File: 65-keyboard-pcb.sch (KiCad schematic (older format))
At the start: 67 parts

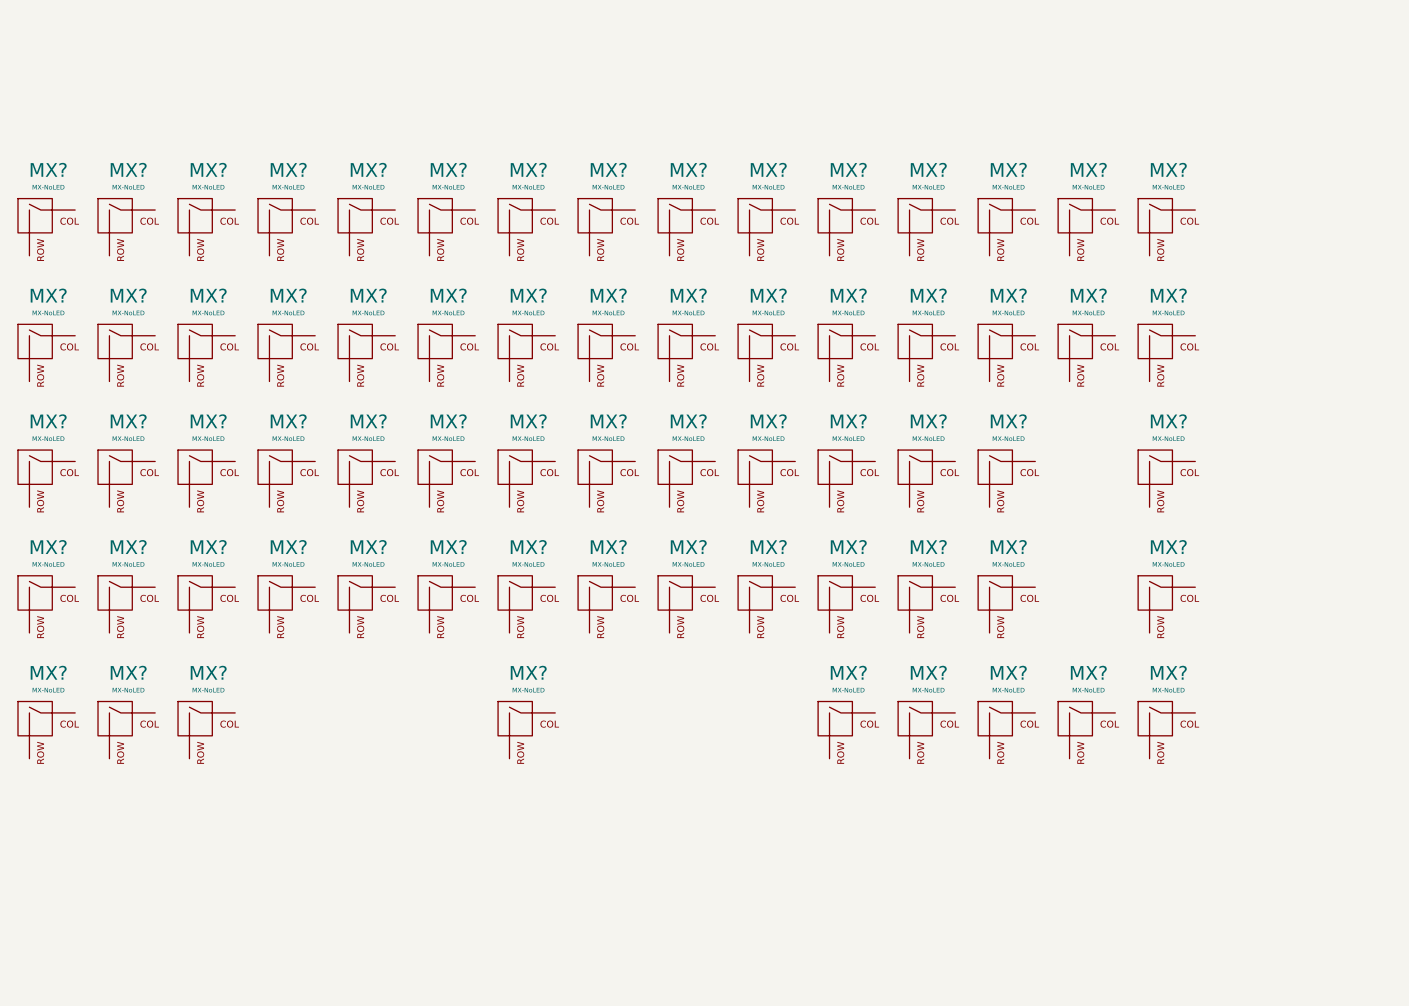
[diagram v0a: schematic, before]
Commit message: Design matrix
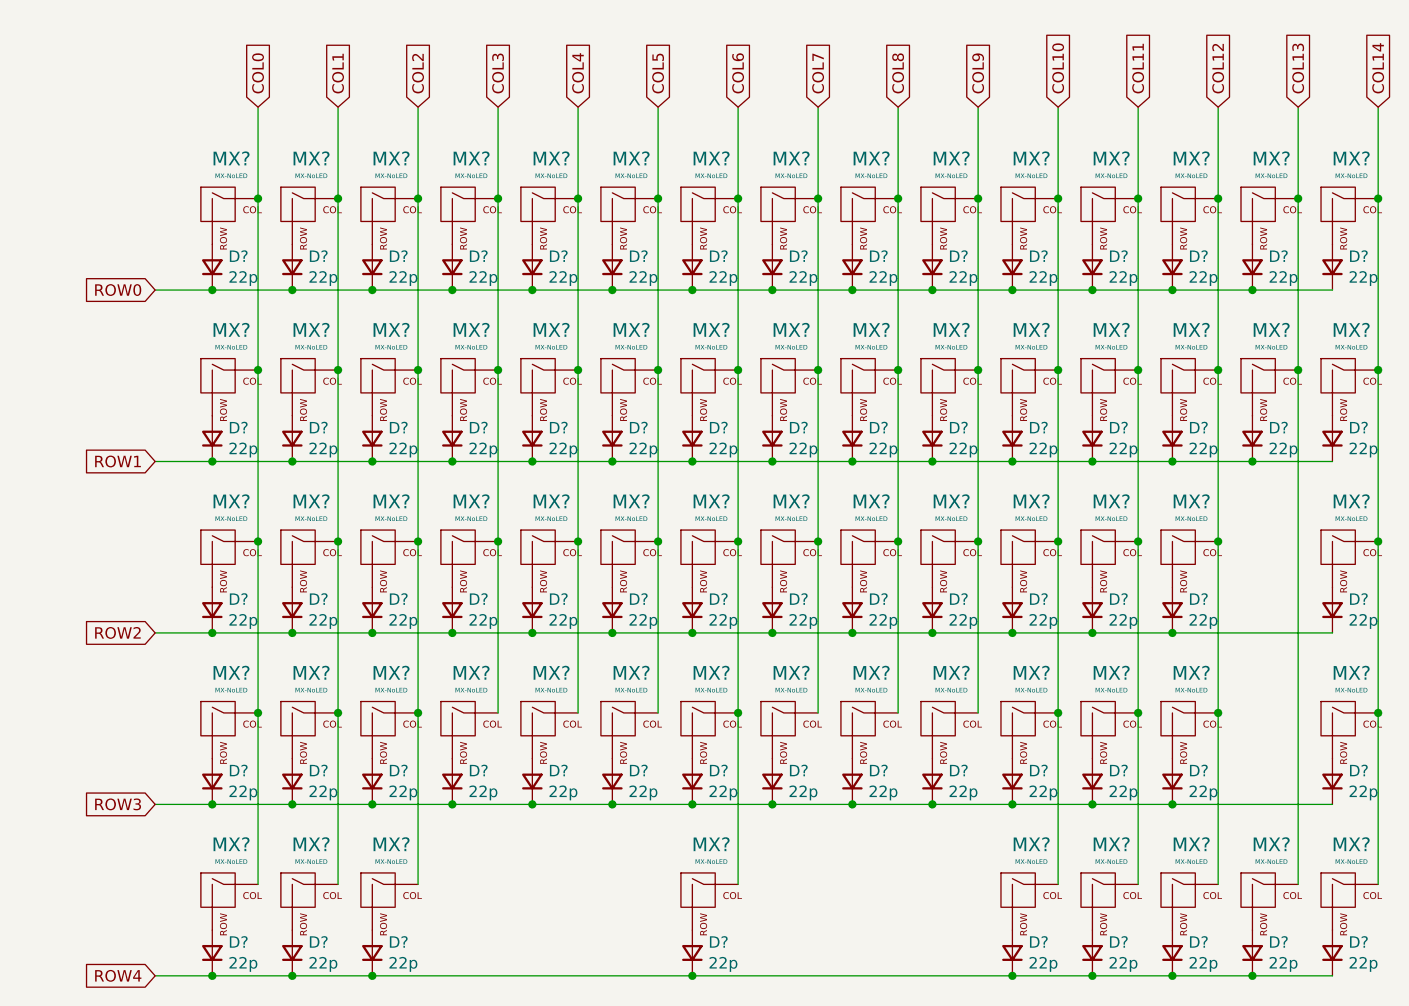
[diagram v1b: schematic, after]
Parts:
- added D? (x67): 22p, symbol Device:D_Small
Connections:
- net COL3: now reaches MX?.1 (COL)
- net COL3: now also MX?.1 (COL), MX?.1 (COL), MX?.1 (COL)
- net at MX?.2 (ROW): now also D?.2 (A) (x67)
- net COL4: now reaches MX?.1 (COL)
- net COL4: now also MX?.1 (COL), MX?.1 (COL), MX?.1 (COL)
- net COL5: now reaches MX?.1 (COL)
- net COL5: now also MX?.1 (COL), MX?.1 (COL), MX?.1 (COL)
- net COL6: now reaches MX?.1 (COL)
- net COL6: now also MX?.1 (COL), MX?.1 (COL), MX?.1 (COL), MX?.1 (COL)
- net COL7: now reaches MX?.1 (COL)
- net COL7: now also MX?.1 (COL), MX?.1 (COL), MX?.1 (COL)
- net COL8: now reaches MX?.1 (COL)
- net COL8: now also MX?.1 (COL), MX?.1 (COL), MX?.1 (COL)
- net COL9: now reaches MX?.1 (COL)
- net COL9: now also MX?.1 (COL), MX?.1 (COL), MX?.1 (COL)
- net COL10: now reaches MX?.1 (COL)
- net COL10: now also MX?.1 (COL), MX?.1 (COL), MX?.1 (COL), MX?.1 (COL)
- net COL11: now reaches MX?.1 (COL)
- net COL11: now also MX?.1 (COL), MX?.1 (COL), MX?.1 (COL), MX?.1 (COL)
- net COL12: now reaches MX?.1 (COL)
- net COL12: now also MX?.1 (COL), MX?.1 (COL), MX?.1 (COL), MX?.1 (COL)
- net COL13: now reaches MX?.1 (COL)
- net COL13: now also MX?.1 (COL), MX?.1 (COL)
- net COL14: now reaches MX?.1 (COL)
- net COL14: now also MX?.1 (COL), MX?.1 (COL), MX?.1 (COL), MX?.1 (COL)
- net COL2: now reaches MX?.1 (COL)
- net COL2: now also MX?.1 (COL), MX?.1 (COL), MX?.1 (COL), MX?.1 (COL)
- net COL1: now reaches MX?.1 (COL)
- net COL1: now also MX?.1 (COL), MX?.1 (COL), MX?.1 (COL), MX?.1 (COL)
- net COL0: now reaches MX?.1 (COL)
- net COL0: now also MX?.1 (COL), MX?.1 (COL), MX?.1 (COL), MX?.1 (COL)
- new net ROW0: D?.1 (K), D?.1 (K), D?.1 (K), D?.1 (K), D?.1 (K), D?.1 (K), D?.1 (K), D?.1 (K), D?.1 (K), D?.1 (K), D?.1 (K), D?.1 (K), D?.1 (K), D?.1 (K), D?.1 (K)
- new net ROW1: D?.1 (K), D?.1 (K), D?.1 (K), D?.1 (K), D?.1 (K), D?.1 (K), D?.1 (K), D?.1 (K), D?.1 (K), D?.1 (K), D?.1 (K), D?.1 (K), D?.1 (K), D?.1 (K), D?.1 (K)
- new net ROW2: D?.1 (K), D?.1 (K), D?.1 (K), D?.1 (K), D?.1 (K), D?.1 (K), D?.1 (K), D?.1 (K), D?.1 (K), D?.1 (K), D?.1 (K), D?.1 (K), D?.1 (K), D?.1 (K)
- new net ROW3: D?.1 (K), D?.1 (K), D?.1 (K), D?.1 (K), D?.1 (K), D?.1 (K), D?.1 (K), D?.1 (K), D?.1 (K), D?.1 (K), D?.1 (K), D?.1 (K), D?.1 (K), D?.1 (K)
- new net ROW4: D?.1 (K), D?.1 (K), D?.1 (K), D?.1 (K), D?.1 (K), D?.1 (K), D?.1 (K), D?.1 (K), D?.1 (K)
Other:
- moved on the sheet: MX?

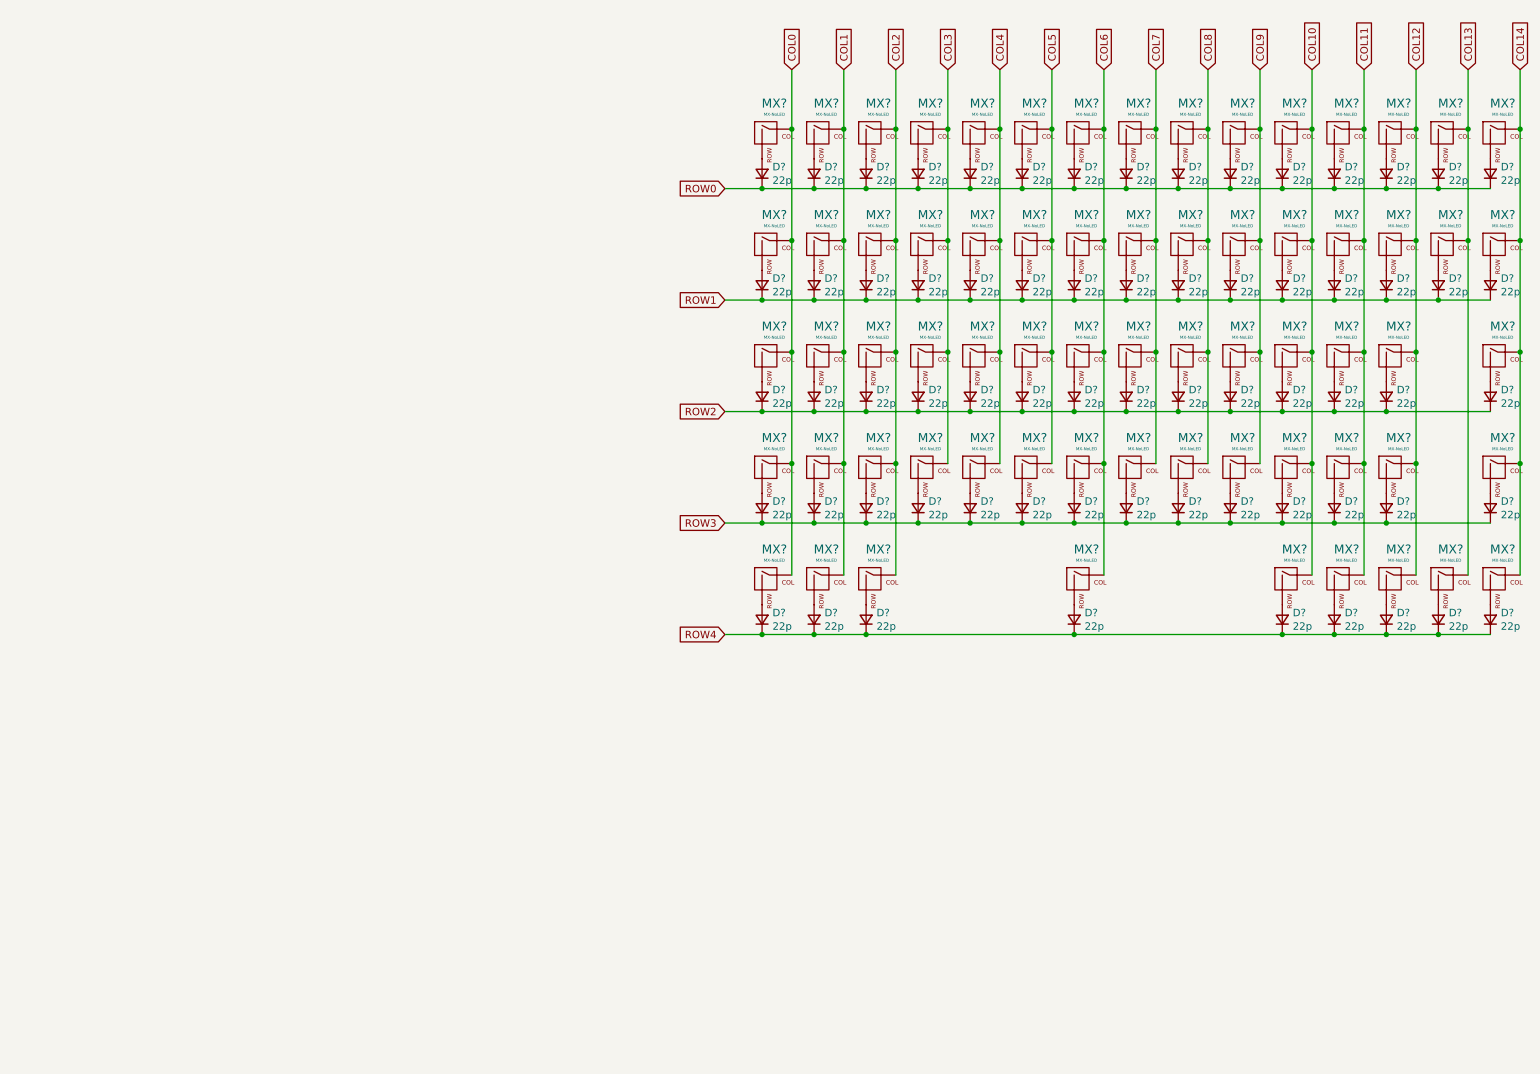
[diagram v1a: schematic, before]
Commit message: Complete schematic
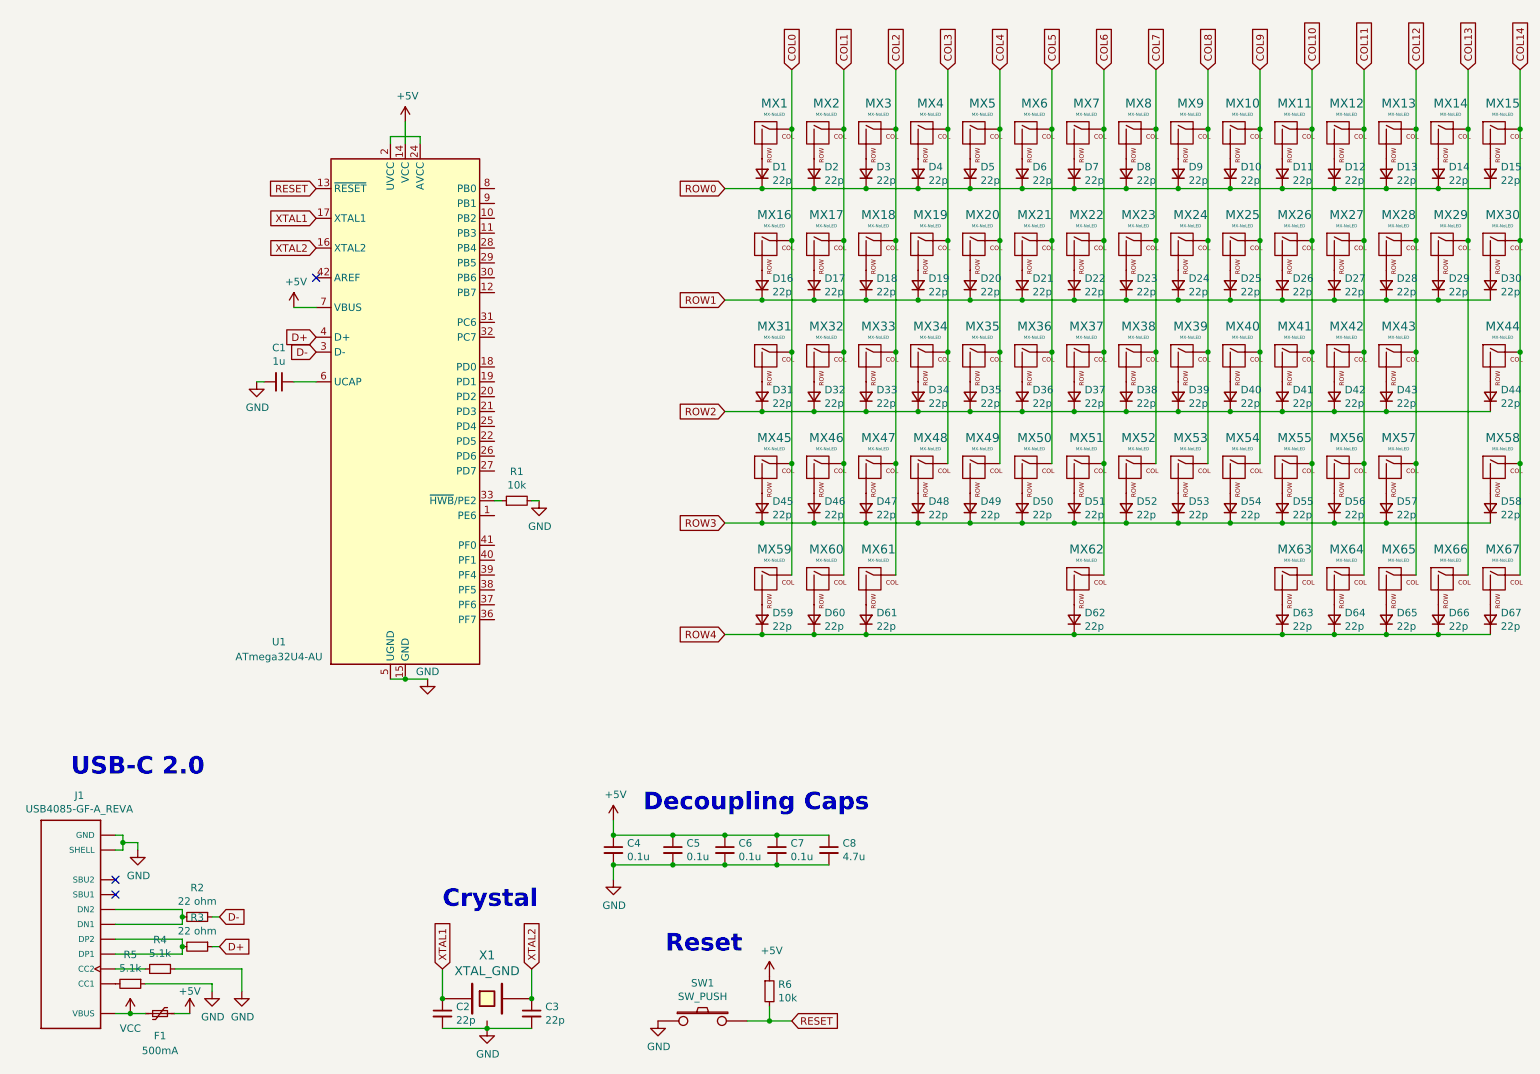
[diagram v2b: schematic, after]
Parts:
- added C1: 1u, Capacitor_SMD:C_0805_2012Metric_Pad1.15x1.40mm_HandSolder, symbol Device:C_Small
- added C2, C3: 22p, Capacitor_SMD:C_0805_2012Metric_Pad1.15x1.40mm_HandSolder, symbol Device:C_Small
- added C4, C5, C6, C7: 0.1u, Capacitor_SMD:C_0805_2012Metric_Pad1.15x1.40mm_HandSolder, symbol Device:C_Small
- added C8: 4.7u, Capacitor_SMD:C_0805_2012Metric_Pad1.15x1.40mm_HandSolder, symbol Device:C_Small
- added F1: 500mA, Fuse:Fuse_1206_3216Metric_Pad1.42x1.75mm_HandSolder, symbol Device:Polyfuse_Small
- added J1: USB4085-GF-A_REVA, USB4085-GF-A_REVA:GCT_USB4085-GF-A_REVA, symbol USB4085-GF-A_REVA:USB4085-GF-A_REVA
- added R1, R6: 10k, Resistor_SMD:R_0805_2012Metric_Pad1.15x1.40mm_HandSolder, symbol Device:R_Small
- added R2, R3: 22 ohm, Resistor_SMD:R_0805_2012Metric_Pad1.15x1.40mm_HandSolder, symbol Device:R_Small
- added R4, R5: 5.1k, Resistor_SMD:R_0805_2012Metric_Pad1.15x1.40mm_HandSolder, symbol Device:R_Small
- added SW1: SW_PUSH, Button_Switch_SMD:SW_SPST_TL3342, symbol keyboard_parts:SW_PUSH
- added U1: ATmega32U4-AU, Package_QFP:TQFP-44_10x10mm_P0.8mm, symbol MCU_Microchip_ATmega:ATmega32U4-AU
- added X1: XTAL_GND, Crystal:Crystal_SMD_SeikoEpson_FA238-4Pin_3.2x2.5mm_HandSoldering, symbol keyboard_parts:XTAL_GND
- D1, D10, D11, D12, D13, D14, D15, D16, D17, D18, D19, D2, D20, D21, D22, D23, D24, D25, D26, D27, D28, D29, D3, D30, D31, D32, D33, D34, D35, D36, D37, D38, D39, D4, D40, D41, D42, D43, D44, D45, D46, D47, D48, D49, D5, D50, D51, D52, D53, D54, D55, D56, D57, D58, D59, D6, D60, D61, D62, D63, D64, D65, D66, D67, D7, D8, D9: renamed from D?; footprint (none) -> Diode_SMD:D_SOD-123
- MX1, MX10, MX11, MX12, MX13, MX15, MX17, MX18, MX19, MX2, MX20, MX21, MX22, MX23, MX24, MX25, MX26, MX27, MX28, MX3, MX30, MX32, MX33, MX34, MX35, MX36, MX37, MX38, MX39, MX4, MX40, MX41, MX42, MX44, MX46, MX47, MX48, MX49, MX5, MX50, MX51, MX52, MX53, MX54, MX55, MX57, MX58, MX6, MX63, MX64, MX65, MX66, MX67, MX7, MX8, MX9: renamed from MX?; footprint (none) -> MX_Only:MXOnly-1U-NoLED
- MX14: renamed from MX?; footprint (none) -> MX_Only:MXOnly-2U-NoLED
- MX16, MX29: renamed from MX?; footprint (none) -> MX_Only:MXOnly-1.5U-NoLED
- MX31, MX59, MX60, MX61: renamed from MX?; footprint (none) -> MX_Only:MXOnly-1.25U-NoLED
- MX43, MX45: renamed from MX?; footprint (none) -> MX_Only:MXOnly-2.25U-NoLED
- MX56: renamed from MX?; footprint (none) -> MX_Only:MXOnly-1.75U-NoLED
- MX62: renamed from MX?; footprint (none) -> MX_Only:MXOnly-7U-ReversedStabilizers-NoLED
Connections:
- new net: U1.2 (UVCC), U1.24 (AVCC), U1.44 (AVCC)
- new net: R1.1, U1.33 (~HWB~/PE2)
- new net: C1.1, U1.6 (UCAP)
- new net: J1.A5 (CC1), R5.2
- new net: J1.A6 (DP1), J1.B6 (DP2), R3.2
- new net: J1.A7 (DN1), J1.B7 (DN2), R2.2
- new net: J1.B5 (CC2), R4.2
- new net +5V: C4.1, C5.1, C6.1, C7.1, C8.1, F1.2, R6.1, U1.14 (VCC), U1.34 (VCC), U1.7 (VBUS)
- new net D+: R3.1, U1.4 (D+)
- new net D-: R2.1, U1.3 (D-)
- new net GND: C1.2, C2.2, C3.2, C4.2, C5.2, C6.2, C7.2, C8.2, J1.A1 (GND), J1.A12 (GND), J1.B1 (GND), J1.B12 (GND), J1.P1 (SHELL), J1.P2 (SHELL), J1.P3 (SHELL), J1.P4 (SHELL), R1.2, R4.1, R5.1, SW1.1, U1.15 (GND), U1.23 (GND), U1.35 (GND), U1.43 (GND), U1.5 (UGND), X1.3
- new net RESET: R6.2, SW1.2, U1.13 (~RESET)
- new net VCC: F1.1, J1.A4 (VBUS), J1.A9 (VBUS), J1.B4 (VBUS), J1.B9 (VBUS)
- new net XTAL1: C2.1, U1.17 (XTAL1), X1.1
- new net XTAL2: C3.1, U1.16 (XTAL2), X1.2
- no-connect marks 0 -> 3
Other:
- note added: "Crystal"
- note added: "Decoupling Caps"
- note added: "Reset\n"
- note added: "USB-C 2.0\n\n"

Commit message: Place components
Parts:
- MX63: footprint MX_Only:MXOnly-1U-NoLED -> MX_Only:MXOnly-1.25U-NoLED
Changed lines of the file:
@@
 F 0 "MX63" H 9433 4623 60  0000 C CNN
 F 1 "MX-NoLED" H 9433 4549 20  0000 C CNN
-F 2 "MX_Only:MXOnly-1U-NoLED" H 8775 4375 60  0001 C CNN
+F 2 "MX_Only:MXOnly-1.25U-NoLED" H 8775 4375 60  0001 C CNN
 F 3 "" H 8775 4375 60  0001 C CNN
 	1    9400 4400
@@
 Wire Wire Line
 	10400 2500 10050 2500
-Wire Wire Line
-	10750 3250 10050 3250
 Connection ~ 5850 3250
 Wire Wire Line
@@
 Wire Wire Line
 	9700 3250 9350 3250
-Connection ~ 10050 3250
-Wire Wire Line
-	10050 3250 9700 3250
-Wire Wire Line
-	10750 4000 10050 4000
 Connection ~ 5850 4000
 Wire Wire Line
@@
 Wire Wire Line
 	9700 4000 9350 4000
-Connection ~ 10050 4000
-Wire Wire Line
-	10050 4000 9700 4000
 Wire Wire Line
 	10750 4750 10400 4750
@@
 Wire Wire Line
 	9900 3600 9900 2850
-Wire Wire Line
-	10250 4350 10250 3600
 Connection ~ 10250 1350
 Wire Wire Line
@@
 Wire Wire Line
 	10250 2100 10250 1350
-Connection ~ 10250 2850
-Wire Wire Line
-	10250 2850 10250 2100
-Connection ~ 10250 3600
-Wire Wire Line
-	10250 3600 10250 2850
-Wire Wire Line
-	10600 4350 10600 2100
 Connection ~ 10600 1350
 Wire Wire Line
@@
 	1    0    0    -1
 $EndComp
+Wire Wire Line
+	10250 2100 10250 2850
+Wire Wire Line
+	9700 4000 10050 4000
+Wire Wire Line
+	9700 3250 10050 3250
+Connection ~ 10250 2850
+Wire Wire Line
+	10250 2850 10250 3600
+Connection ~ 10050 3250
+Connection ~ 10250 3600
+Wire Wire Line
+	10250 3600 10250 4350
+Connection ~ 10050 4000
+Wire Wire Line
+	10050 3250 10750 3250
+Wire Wire Line
+	10050 4000 10750 4000
+Wire Wire Line
+	10600 2100 10600 4350
 $EndSCHEMATC
